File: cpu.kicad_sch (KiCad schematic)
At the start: 30 parts, among them J81 Conn_01x03_Pin, J82 Conn_Coaxial, J83 Conn_Coaxial, J84 Conn_01x02_Pin, SW81 SW_Push, SW82 SW_Push, U8 ESP32-C6-MINI-1U, U81 74HC595, U82 74HC595, U83 74HC595, U84 ISOW7842

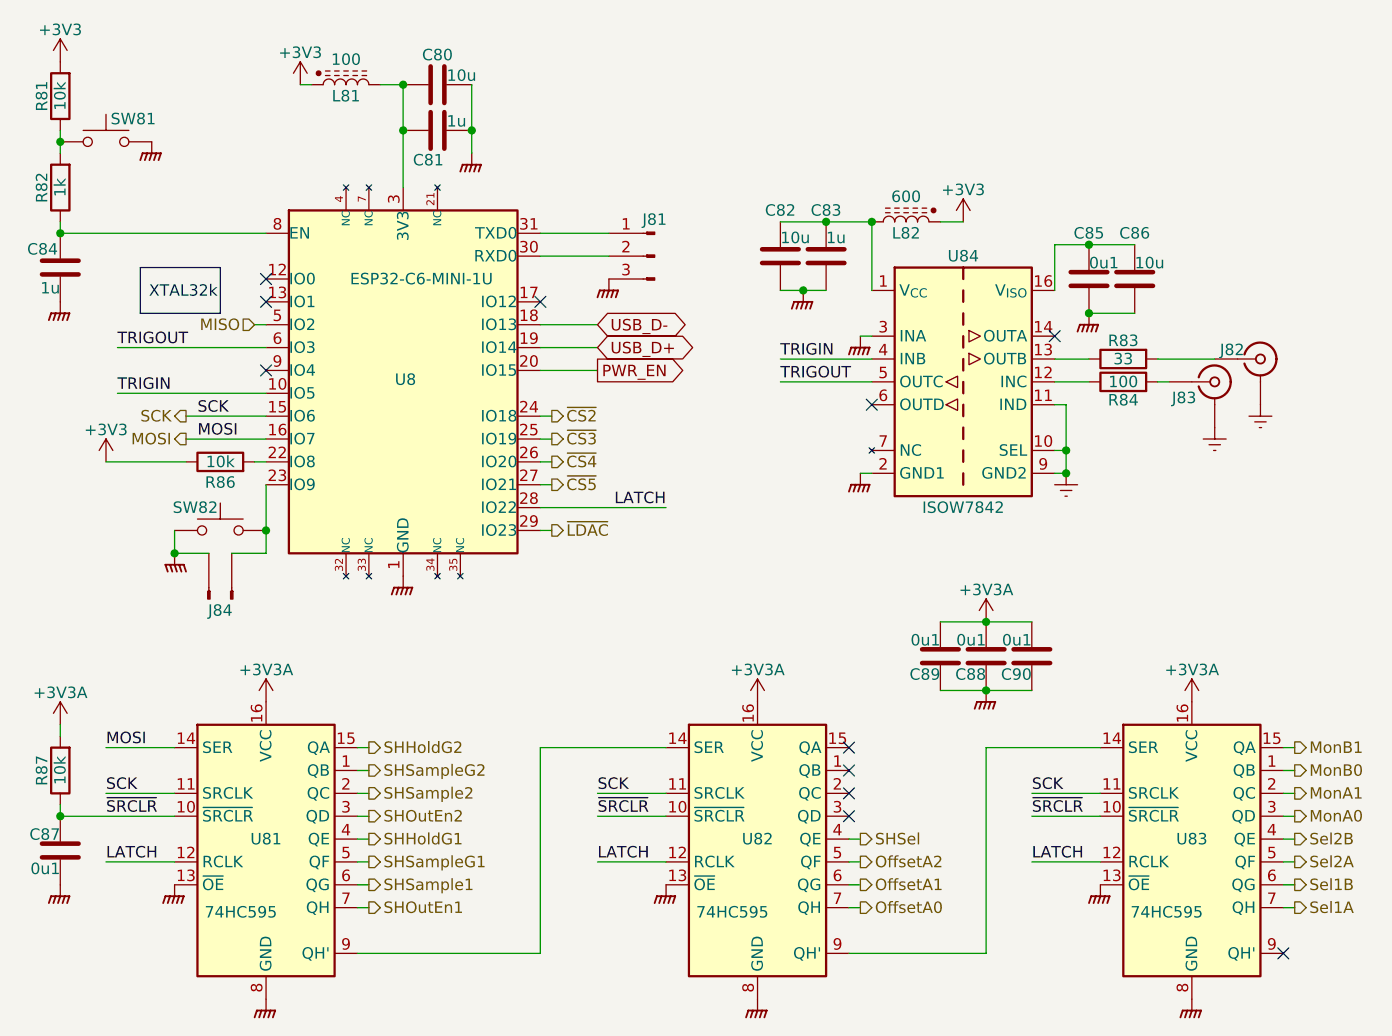
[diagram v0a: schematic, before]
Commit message: Scan deleted.
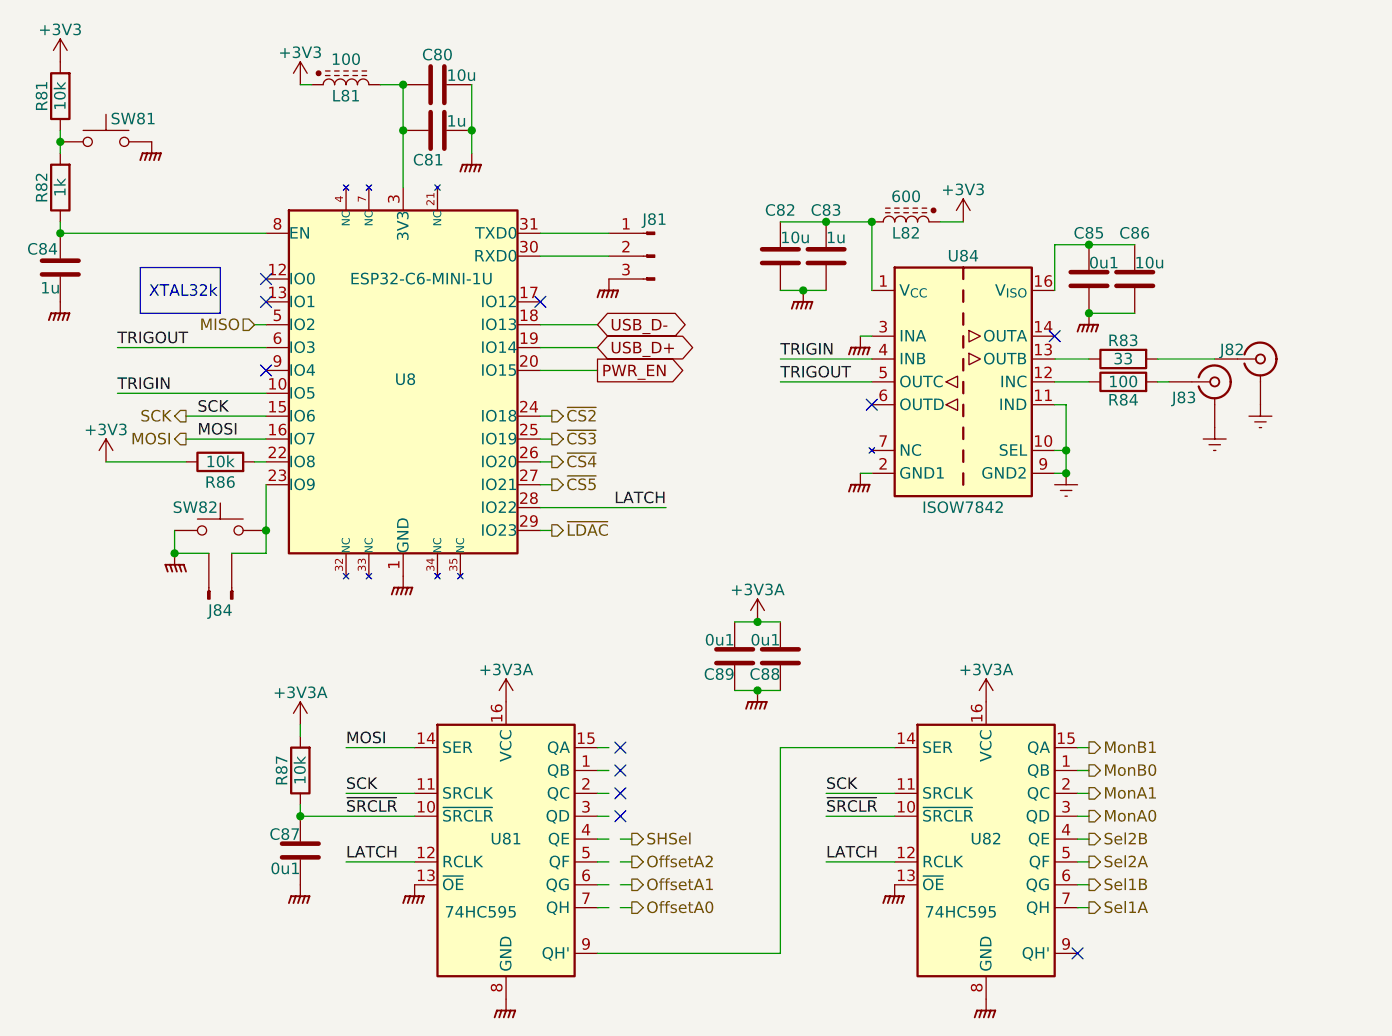
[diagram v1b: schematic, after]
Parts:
- removed C90: 0u1, Capacitor_SMD:C_0402_1005Metric, symbol Device:C
- removed U83: 74HC595, Package_SO:SOIC-16_3.9x9.9mm_P1.27mm, symbol 74xx:74HC595
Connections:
- net MonA0: now also U82.3 (QD)
- net MonA1: now also U82.2 (QC)
- net MonB0: now also U82.1 (QB)
- net MonB1: now also U82.15 (QA)
- net OffsetA0: no longer U82.7 (QH)
- net OffsetA1: no longer U82.6 (QG)
- net OffsetA2: no longer U82.5 (QF)
- net SHSel: no longer U82.4 (QE)
- net Sel1A: now also U82.7 (QH)
- net Sel1B: now also U82.6 (QG)
- net Sel2A: now also U82.5 (QF)
- net Sel2B: now also U82.4 (QE)
- net SHHoldG1: no longer names the net of U81.4 (QE)
- net SHHoldG2: no longer names the net of U81.15 (QA)
- net SHOutEn1: no longer names the net of U81.7 (QH)
- net SHOutEn2: no longer names the net of U81.3 (QD)
- net SHSample1: no longer names the net of U81.6 (QG)
- net SHSample2: no longer names the net of U81.2 (QC)
- net SHSampleG1: no longer names the net of U81.5 (QF)
- net SHSampleG2: no longer names the net of U81.1 (QB)
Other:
- moved on the sheet: C87, C88, C89, R87, U81, U82

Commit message: Most blocks there....
About to restore scan.
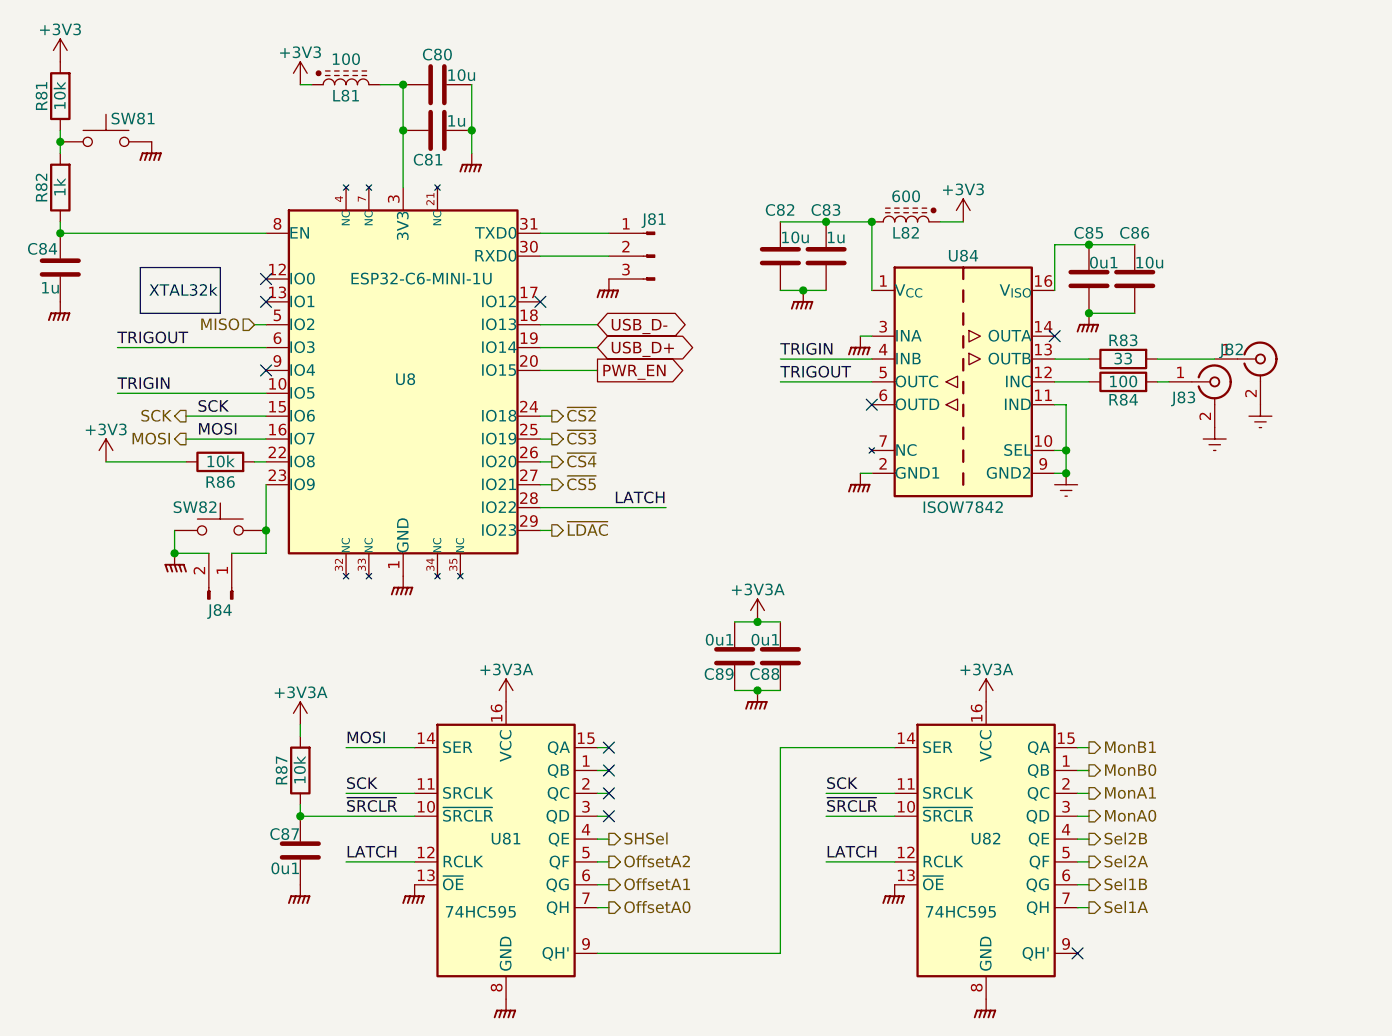
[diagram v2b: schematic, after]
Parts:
- R83: footprint Resistor_SMD:R_0603_1608Metric -> Resistor_SMD:R_0402_1005Metric; LCSC C23140 -> C25105
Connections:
- net OffsetA0: now also U81.7 (QH)
- net OffsetA1: now also U81.6 (QG)
- net OffsetA2: now also U81.5 (QF)
- net SHSel: now also U81.4 (QE)
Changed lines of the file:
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@@
 	)
 	(no_connect
-		(at 119.38 107.95)
+		(at 118.11 107.95)
 	)
 	(no_connect
@@
 	)
 	(no_connect
-		(at 119.38 113.03)
+		(at 118.11 113.03)
 	)
 	(no_connect
@@
 	)
 	(no_connect
-		(at 119.38 105.41)
+		(at 118.11 105.41)
 	)
 	(no_connect
@@
 	)
 	(no_connect
-		(at 119.38 110.49)
+		(at 118.11 110.49)
 	)
 	(no_connect
@@
 	(wire
 		(pts
-			(xy 119.38 123.19) (xy 120.65 123.19)
-		)
-		(stroke
-			(width 0)
-			(type default)
-		)
-	)
-	(wire
-		(pts
-			(xy 119.38 118.11) (xy 120.65 118.11)
-		)
-		(stroke
-			(width 0)
-			(type default)
-		)
-	)
-	(wire
-		(pts
 			(xy 170.18 115.57) (xy 171.45 115.57)
 		)
@@
 	(wire
 		(pts
-			(xy 119.38 115.57) (xy 120.65 115.57)
-		)
-		(stroke
-			(width 0)
-			(type default)
-		)
-	)
-	(wire
-		(pts
 			(xy 57.15 48.26) (xy 80.01 48.26)
 		)
@@
 	(wire
 		(pts
-			(xy 119.38 120.65) (xy 120.65 120.65)
-		)
-		(stroke
-			(width 0)
-			(type default)
-		)
-	)
-	(wire
-		(pts
 			(xy 71.12 71.12) (xy 80.01 71.12)
 		)
@@
 	(hierarchical_label "OffsetA0"
 		(shape output)
-		(at 120.65 123.19 0)
+		(at 118.11 123.19 0)
 		(effects
 			(font
@@
 	(hierarchical_label "SHSel"
 		(shape output)
-		(at 120.65 115.57 0)
+		(at 118.11 115.57 0)
 		(effects
 			(font
@@
 	(hierarchical_label "OffsetA2"
 		(shape output)
-		(at 120.65 118.11 0)
+		(at 118.11 118.11 0)
 		(effects
 			(font
@@
 	(hierarchical_label "OffsetA1"
 		(shape output)
-		(at 120.65 120.65 0)
+		(at 118.11 120.65 0)
 		(effects
 			(font
@@
 	)
 	(symbol
-		(lib_name "Conn_Coaxial_1")
 		(lib_id "Connector:Conn_Coaxial")
 		(at 190.5 62.23 0)
@@
 			)
 		)
-		(property "Footprint" "Resistor_SMD:R_0603_1608Metric"
+		(property "Footprint" "Resistor_SMD:R_0402_1005Metric"
 			(at 175.26 60.452 90)
 			(effects
@@
 			)
 		)
-		(property "LCSC" "C23140"
+		(property "LCSC" "C25105"
 			(at 175.26 62.23 90)
 			(effects
